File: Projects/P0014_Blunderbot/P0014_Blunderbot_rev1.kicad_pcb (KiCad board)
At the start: 2 copper layers, 63.5 x 25.4 mm, 19 parts, among them J1 22-03-5035, J2 22-03-5035, J3 70553-0037, J4 70553-0037, J5 CONN_01X04, J6 CONN_01X04, P1 CONN_02X03, U1 TC7W241FUTE12LF, U2 MIC5219-5.0YM5-TR, U3 MIC5219-5.0YM5-TR, U4 ATTINY841-SSU

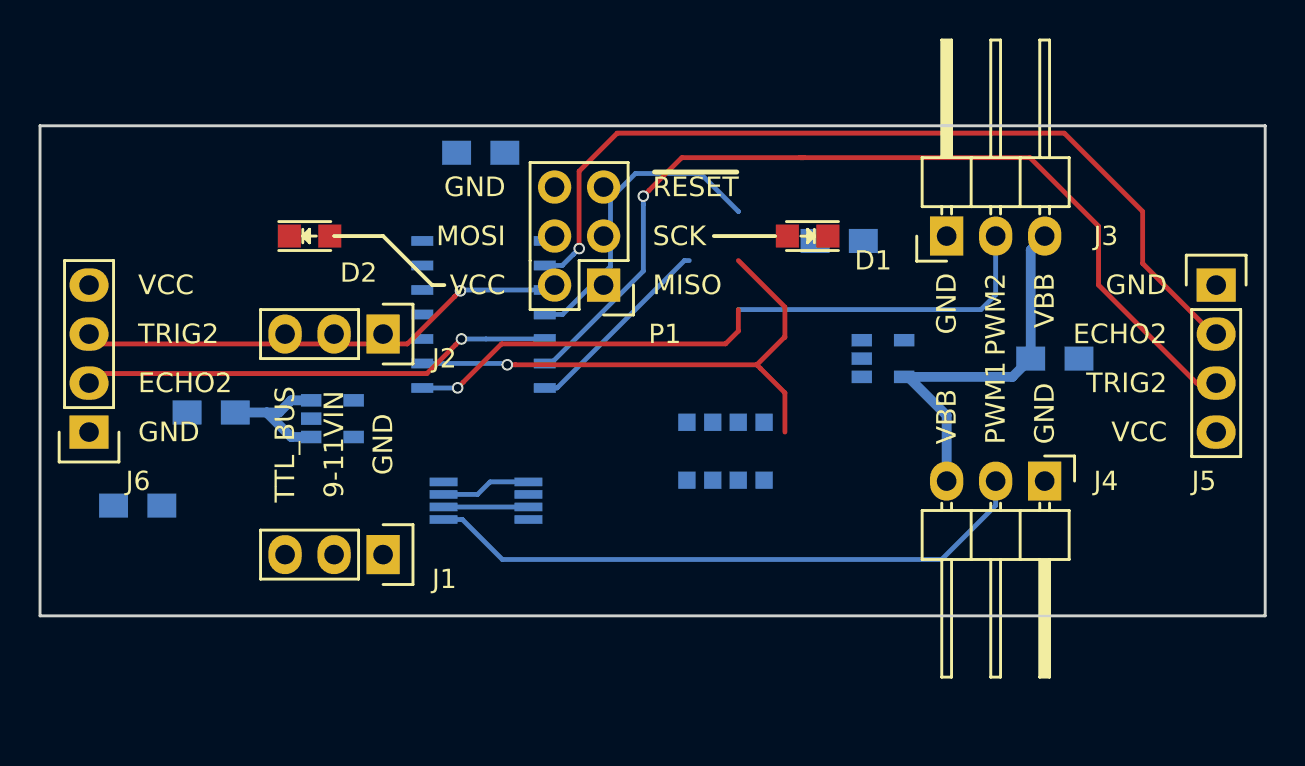
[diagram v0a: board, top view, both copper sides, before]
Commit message: layout nearly done
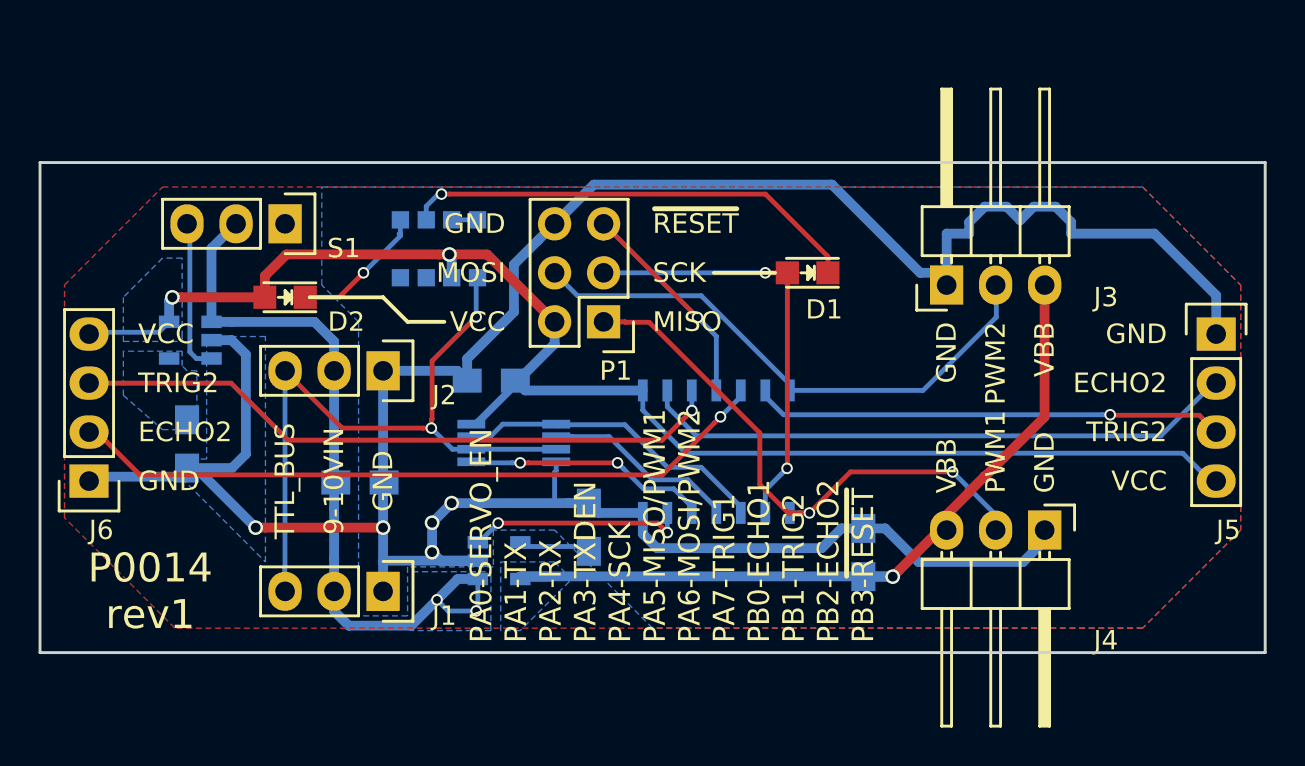
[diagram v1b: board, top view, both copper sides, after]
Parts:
- added S1: MHSS1105, Pin_Headers:Pin_Header_Straight_1x03, F.Cu at (129.5, 89.5)
- moved U3 22.5 mm to (140.6, 107.0)
- moved C2 19.7 mm to (145.3, 105.3), turned to 90 degrees
- moved RP1 18.2 mm to (137.5, 90.8)
- moved U4 14.2 mm to (151.9, 101.5), turned to 0 degrees
- moved C4 14.1 mm to (159.5, 106.6), turned to 90 degrees
- moved C5 11.8 mm to (140.2, 97.7)
- moved C1 8.52 mm to (133.4, 102.9), turned to 0 degrees
- moved U2 8.42 mm to (124.6, 95.6), turned to 180 degrees
- moved C3 4.09 mm to (124.5, 100.9), turned to 270 degrees
- moved D2 3.42 mm to (129.5, 93.3), turned to 180 degrees
- moved U1 3.32 mm to (141.4, 100.9)
- moved J5 2.54 mm to (177.8, 95.2)
- moved J6 2.54 mm to (119.4, 102.9)
- moved J3 2.54 mm to (163.8, 92.7)
- moved J4 2.54 mm to (168.9, 105.4)
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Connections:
- C1 pad 1: /9-12V_IN -> /9-10V_IN
- J1 pad 2: /9-12V_IN -> /9-10V_IN
- J2 pad 2: /9-12V_IN -> /9-10V_IN
- J3 pad 2: /MISO -> /MOSI/PWM2
- J4 pad 2: /PWM1 -> /MISO/PWM1
- P1 pad 1: /MISO -> /MISO/PWM1
- P1 pad 4: /MOSI -> /MOSI/PWM2
- U1 pad 5: /PWM1 -> /TX
- U2 pad 1: /9-12V_IN -> /9-10V_IN
- U2 pad 3: /9-12V_IN -> Net-(S1-Pad3)
- U3 pad 1: /9-12V_IN -> /9-10V_IN
- U4 pad 10: /SERVO_EN -> /TXDEN
- U4 pad 12: /PWM1 -> /TX
- U4 pad 13: /TXDEN -> /SERVO_EN
- U4 pad 7: /MOSI -> /MOSI/PWM2
- U4 pad 8: /MISO -> /MISO/PWM1
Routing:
- net GND: track 0.00 -> 148.0 mm, vias 0 -> 5
- net /VCC: track 4.39 -> 76.6 mm, vias 0 -> 2
- net /9-10V_IN: track 0.00 -> 40.6 mm, vias 0 -> 2
- net /MISO: track 35.4 -> 0.00 mm, vias 1 -> 0
- net /PWM1: track 31.9 -> 0.00 mm
- net /TTL_BUS: track 4.40 -> 36.3 mm, vias 0 -> 2
- net /MOSI/PWM2: track 0.00 -> 29.4 mm
- net /MISO/PWM1: track 0.00 -> 29.1 mm, vias 0 -> 2
- net Net-(D1-Pad1): track 0.00 -> 24.0 mm, vias 0 -> 1
- net /TRIG1: track 48.4 -> 24.5 mm
- net /VBB: track 20.0 -> 41.5 mm, vias 0 -> 1
- net /TRIG2: track 20.6 -> 33.7 mm
- net /TX: track 0.00 -> 12.6 mm, vias 0 -> 2
- net /ECHO2: track 24.6 -> 37.1 mm
- net /TXDEN: track 4.67 -> 16.9 mm
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- added copper zone on B.Cu, net /9-10V_IN
- added copper zone on B.Cu, net /VBB
- added copper zone on B.Cu, net /VCC
- added copper zone on B.Cu, net GND
- added copper zone on F.Cu, net GND
- added copper zone on B.Cu, net Net-(C3-Pad1)
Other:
- board text added: "9-10VIN"
- board text added: "Blunderbot"
- board text added: "Designed by Max Prokopenko"
- board text added: "OpenRobotics.ca"
- board text added: "P0014 rev1"
- board text added: "PA0-SERVO_EN PA1-TX PA2-RX PA3-TXDEN PA4-SCK PA5-MISO/PWM1 PA6-MOSI/PWM2 PA7-TRIG1 PB0-ECHO1 PB1-TRIG2 PB2-ECHO2 PB3-~RESET"
- board text removed: "9-11VIN"
